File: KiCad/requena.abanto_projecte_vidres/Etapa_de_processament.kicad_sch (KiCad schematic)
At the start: 45 parts, among them J1 Conn_01x05, J2 Conn_01x04_Socket, J3 DE9_Pins, J4 DE9_Pins, SW1 SW_Push_SPDT, SW2 SW_Push, SW3 SW_Omron_B3FS, SW4 SW_Omron_B3FS, SW5 SW_Omron_B3FS, SW6 SW_Omron_B3FS, U10 NMUX1308PW, U7 PN5120A0HN1, U8 PIC24HJ128GP502, U9 TJA1051TK-3, Y1 27.12 MHz, Y2 8 MHz

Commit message: Millora del micro a 44 pins
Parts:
- removed C22: 100n, Capacitor_SMD:C_1206_3216Metric, symbol Device:C
- removed U10: NMUX1308PW, Package_SO:TSSOP-16_4.4x5mm_P0.65mm, symbol Analog_Switch:NMUX1308PW
- removed U8: PIC24HJ128GP502, Package_SO:SSOP-28_5.3x10.2mm_P0.65mm, symbol biblioteca_de_projecte:PIC18F23K20_ISS
- added U6: PIC24HJ128GP502, Package_QFP:TQFP-44_10x10mm_P0.8mm, symbol MCU_Microchip_PIC32:PIC32MX250F128D-IPT
- Y1, Y2: footprint Crystal:Crystal_SMD_HC49-SD -> Crystal:Crystal_SMD_3225-4Pin_3.2x2.5mm
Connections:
- net AN0: now also U6.19 (RA0/ANO)
- net GND: no longer C14.2, C16.2, C18.2, C19.2, J1.3 (Pin_3), J3.5, SW2.2
- net OSC1: now also U6.31 (OSC2)
- net OSC2: now also U6.30 (OSC1)
- net at C17.1: now also U6.7 (VCAP)
- new net: C14.2, C16.2
- new net: C18.2, C19.2, J3.5
- new net: U6.28 (VDD), U6.40 (VDD)
- new net: U6.29 (VSS), U6.39 (VSS), U6.6 (VSS)
- new net: J1.3 (Pin_3), SW2.2
- no-connect marks 22 -> 18
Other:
- note removed: "MUX 8-1"
- moved on the sheet: C10, C11, C12, C13, C14, C15, C16, C17, C7, C8, C9, J2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

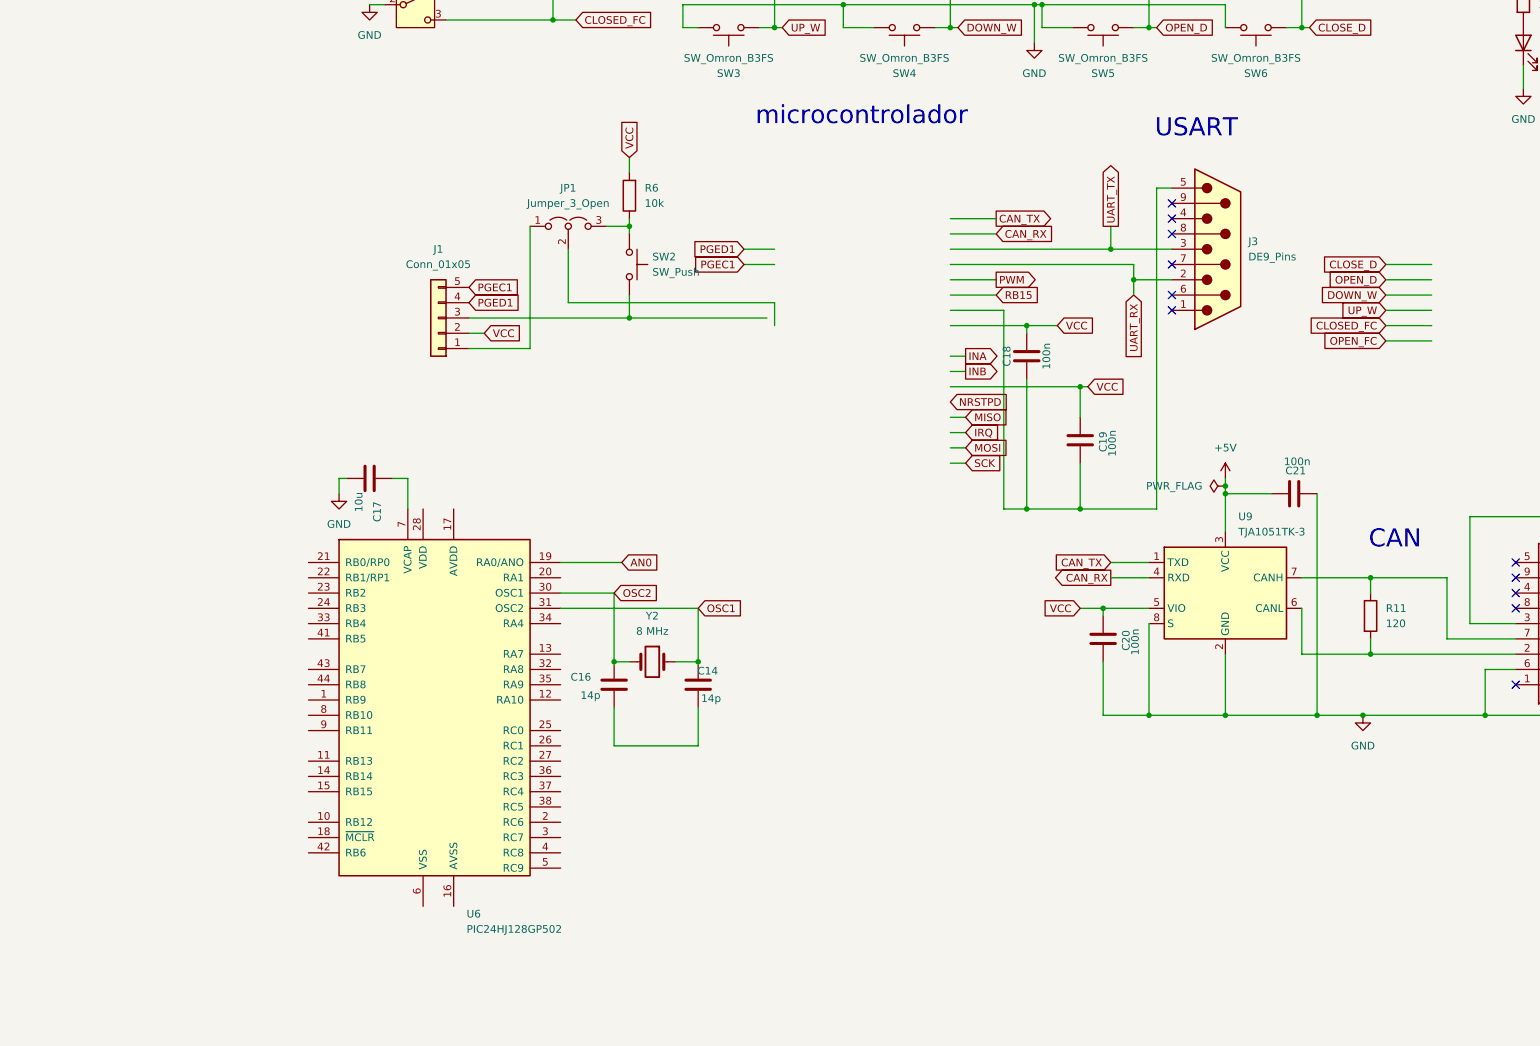
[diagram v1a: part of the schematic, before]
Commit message: .
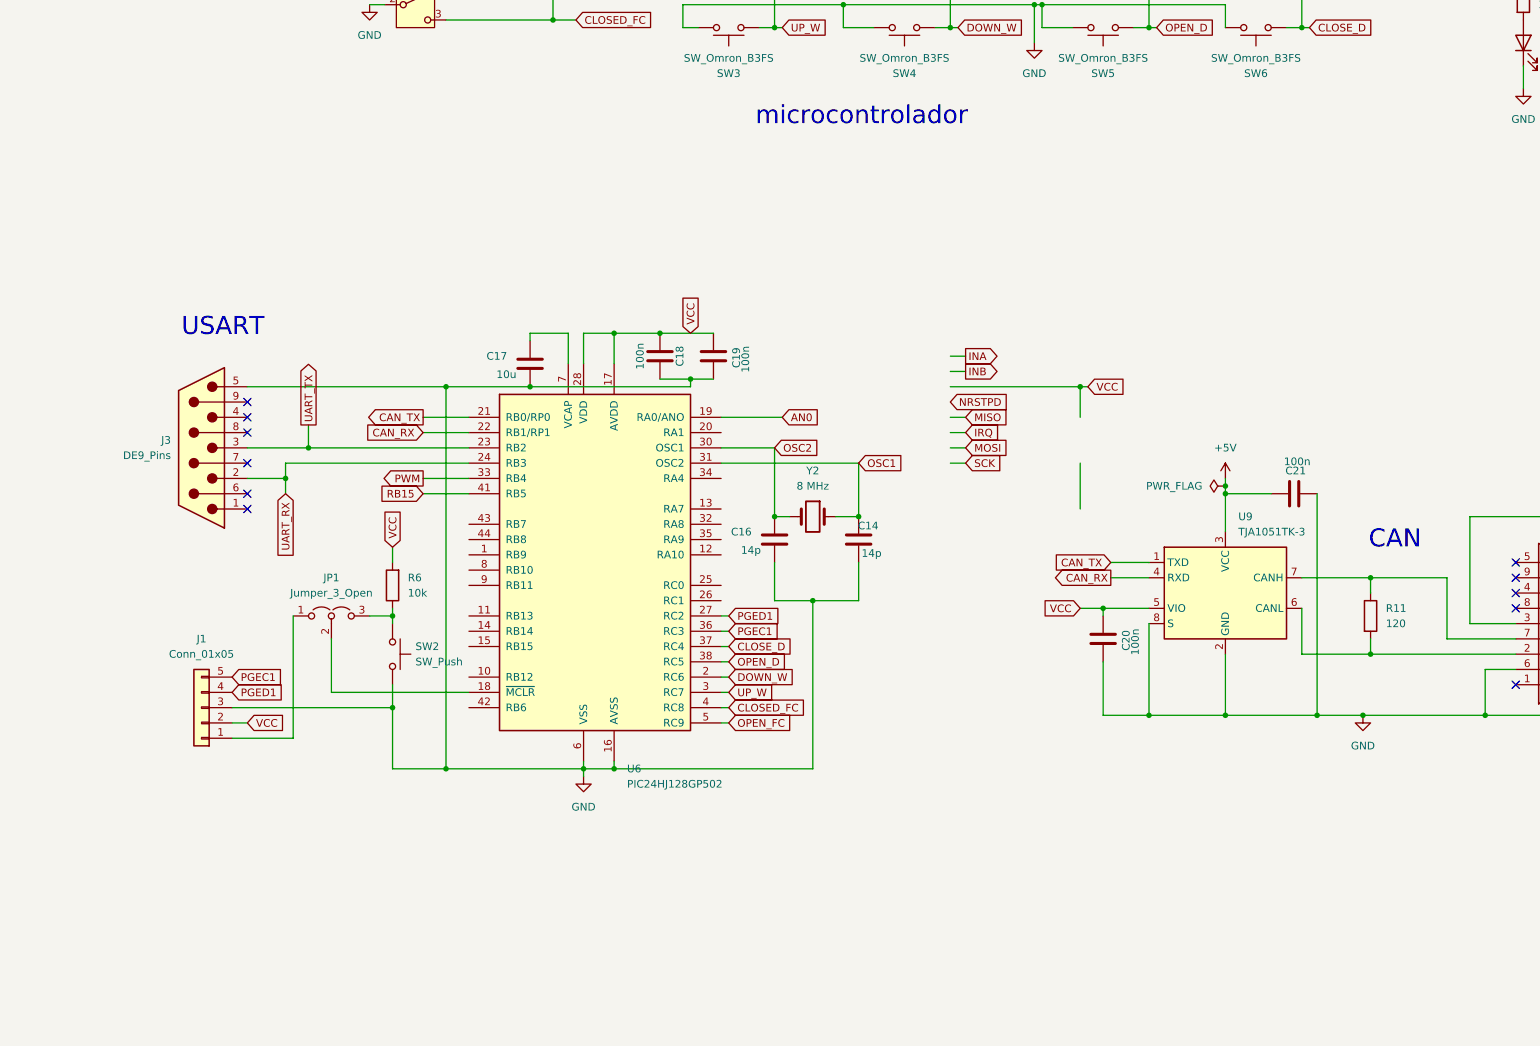
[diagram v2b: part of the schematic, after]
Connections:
- net CAN_RX: now also U6.22 (RB1/RP1)
- net CAN_TX: now also U6.21 (RB0/RP0)
- net CLOSED_FC: now also U6.4 (RC8)
- net CLOSE_D: now also U6.37 (RC4)
- net DOWN_W: now also U6.2 (RC6)
- net GND: now also C14.2, C16.2, C18.1, C19.2, J1.3 (Pin_3), J3.5, SW2.2, U6.16 (AVSS), U6.29 (VSS), U6.39 (VSS), U6.6 (VSS)
- net OPEN_D: now also U6.38 (RC5)
- net OPEN_FC: now also U6.5 (RC9)
- net PGEC1: now also U6.36 (RC3)
- net PGED1: now also U6.27 (RC2)
- net PWM: now also U6.33 (RB4)
- net RB15: now also U6.41 (RB5)
- net UART_RX: now also U6.24 (RB3)
- net UART_TX: now also U6.23 (RB2)
- net UP_W: now also U6.3 (RC7)
- net VCC: now also C18.2, U6.17 (AVDD), U6.28 (VDD), U6.40 (VDD); no longer C18.1
- net at U6.18 (~{MCLR}): now also JP1.2 (C)
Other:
- moved on the sheet: C14, C16, C17, C18, J1, J3, JP1, R6, SW2, U6, Y2

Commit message: esquema acabat
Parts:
- removed J2: Conn_01x04_Socket, Connector_JST:JST_XH_B4B-XH-AM_1x04_P2.50mm_Vertical, symbol Connector:Conn_01x04_Socket
- added J6: Conn_01x04, TerminalBlock:TerminalBlock_Xinya_XY308-2.54-4P_1x04_P2.54mm_Horizontal, symbol Connector_Generic:Conn_01x04
- J3, J4: footprint Connector_Dsub:DSUB-9_Pins_Vertical_P2.77x2.84mm -> Connector_Dsub:DSUB-9_Pins_Horizontal_P2.77x2.84mm_EdgePinOffset4.94mm_Housed_MountingHolesOffset4.94mm
- Y1, Y2: footprint Crystal:Crystal_SMD_3225-4Pin_3.2x2.5mm -> Crystal:Crystal_SMD_3215-2Pin_3.2x1.5mm
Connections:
- net INA: now also U6.13 (RA7)
- net INB: now also U6.32 (RA8)
- net IRQ: now also U6.1 (RB9)
- net MISO: now also U6.44 (RB8)
- net MOSI: now also U6.8 (RB10)
- net NRSTPD: now also U6.43 (RB7)
- net SCK: now also U6.9 (RB11)
- net at U7.19 (AUX1): now also J6.3 (Pin_3)
- net at U7.20 (AUX2): now also J6.4 (Pin_4)
- net at U7.7 (SIGIN): now also J6.1 (Pin_1)
- net at U7.8 (SIGOUT): now also J6.2 (Pin_2)
- no-connect marks 18 -> 29
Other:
- moved on the sheet: C10, C11, C12, C13, C14, C15, C16, C17, C18, C19, C20, C21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
